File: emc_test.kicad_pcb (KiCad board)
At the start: 2 copper layers, 102 x 57 mm, 42 parts, among them X1 NEU, X2 LINE, X3 PE, X4 LINE, X5 PE, X6 NEU

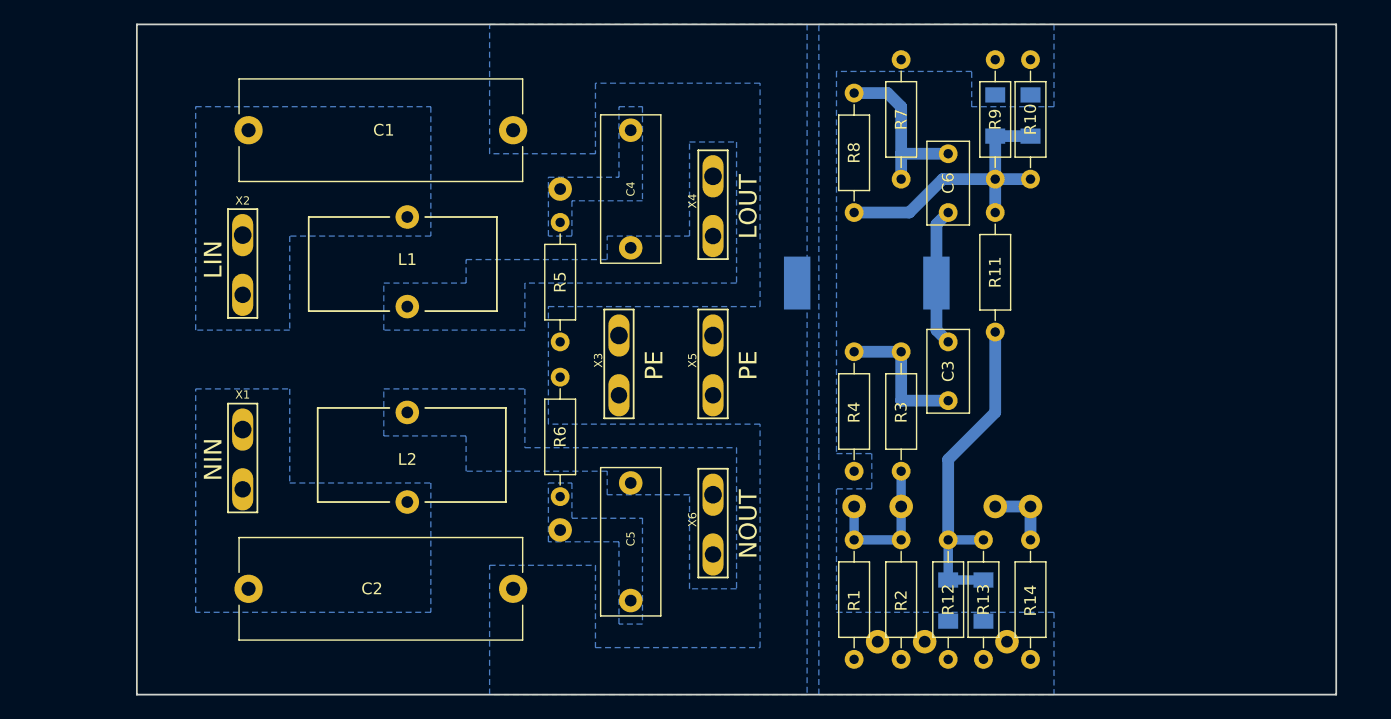
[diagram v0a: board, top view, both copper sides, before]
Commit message: plokstes paruosimas
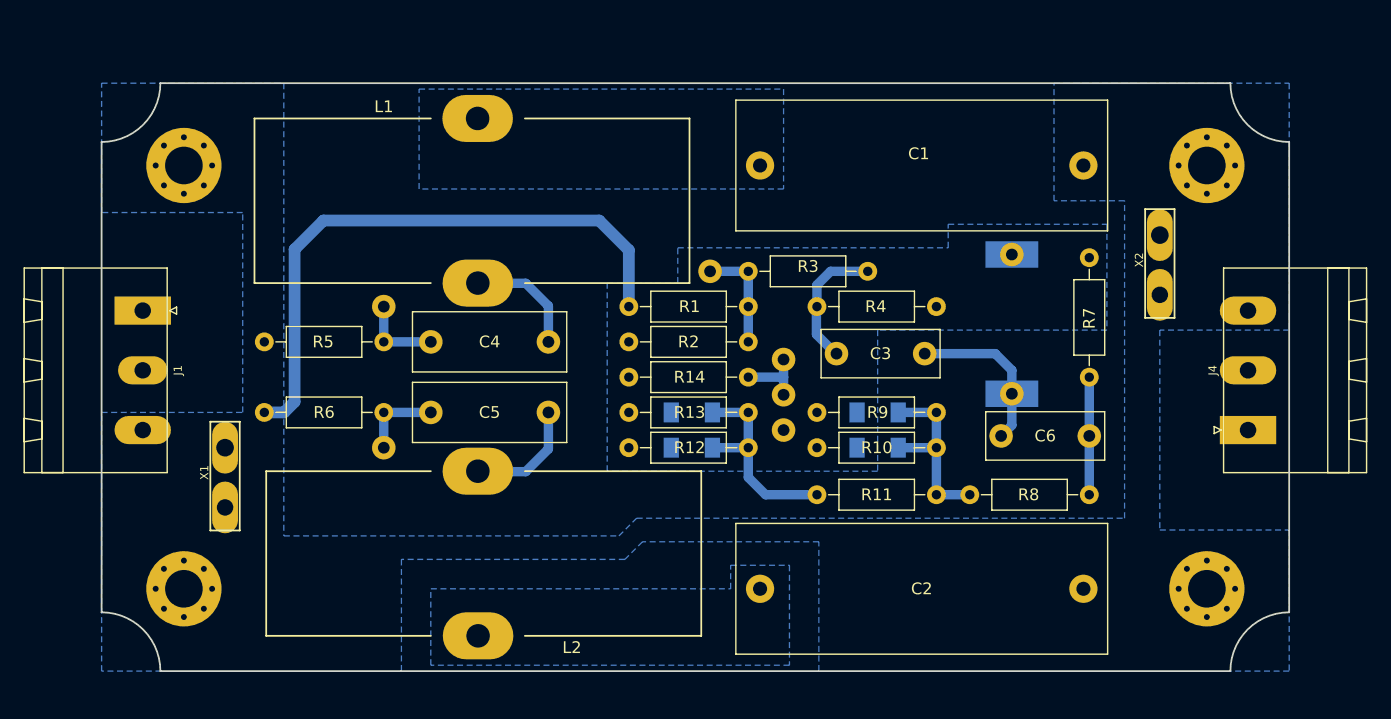
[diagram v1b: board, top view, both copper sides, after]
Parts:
- removed the REF** at (164.0, 121.5)
- removed the REF** at (168.0, 121.5)
- removed the REF** at (175.0, 121.5)
- removed the REF** at (177.0, 110.0)
- removed the REF** at (174.0, 110.0)
- removed the REF** at (162.0, 110.0)
- removed the REF** at (166.0, 110.0)
- removed the REF** at (137.0, 112.0)
- removed the REF** at (137.0, 83.0)
- removed X3, X5: PE, mech:Faston_6.3x0.8x14
- removed X4: LINE, mech:Faston_6.3x0.8x14
- removed X6: NEU, mech:Faston_6.3x0.8x14
- added J1: MSTBA_3C_5.08_Angled, mech:PhoenixContact_MSTBA-G_03x5.08mm_Angled, F.Cu at (101.5, 93.3)
- added J4: MSTBA_3C_5.08_Angled, mech:PhoenixContact_MSTBA-G_03x5.08mm_Angled, F.Cu at (195.5, 103.5)
- added REF**: SolderWirePad_single_1mmDrill, Wire_Pads:SolderWirePad_single_1mmDrill, F.Cu at (149.8, 90.0)
- added REF**: MountingHole_3.2mm_M3_Pad_Via, Mounting_Holes:MountingHole_3.2mm_M3_Pad_Via, F.Cu at (192.0, 81.0)
- added REF**: MountingHole_3.2mm_M3_Pad_Via, Mounting_Holes:MountingHole_3.2mm_M3_Pad_Via, F.Cu at (105.0, 117.0)
- added REF**: MountingHole_3.2mm_M3_Pad_Via, Mounting_Holes:MountingHole_3.2mm_M3_Pad_Via, F.Cu at (105.0, 81.0)
- added REF**: SolderWirePad_single_1mmDrill, Wire_Pads:SolderWirePad_single_1mmDrill, F.Cu at (156.0, 103.5)
- added REF**: SolderWirePad_single_1mmDrill, Wire_Pads:SolderWirePad_single_1mmDrill, F.Cu at (156.0, 100.5)
- added REF**: SolderWirePad_single_1mmDrill, Wire_Pads:SolderWirePad_single_1mmDrill, F.Cu at (156.0, 97.5)
- added REF**: SolderWirePad_single_1mmDrill, Wire_Pads:SolderWirePad_single_1mmDrill, F.Cu at (122.0, 105.0)
- added REF**: SolderWirePad_single_1mmDrill, Wire_Pads:SolderWirePad_single_1mmDrill, F.Cu at (122.0, 93.0)
- added REF**: SolderWirePad_single_1mmDrill, Wire_Pads:SolderWirePad_single_1mmDrill, F.Cu at (175.4, 100.4)
- added REF**: SolderWirePad_single_1mmDrill, Wire_Pads:SolderWirePad_single_1mmDrill, F.Cu at (175.4, 88.6)
- added REF**: MountingHole_3.2mm_M3_Pad_Via, Mounting_Holes:MountingHole_3.2mm_M3_Pad_Via, F.Cu at (192.0, 117.0)
- C1, C2: footprint Capacitors_THT:C_Rect_L24.0mm_W8.6mm_P22.50mm_MKT -> Capacitors_THT:C_Rect_L31.5mm_W11.0mm_P27.50mm_MKS4
- C3, C6: footprint Capacitors_THT:C_Rect_L7.0mm_W3.5mm_P5.00mm -> Capacitors_THT:C_Rect_L10.0mm_W4.0mm_P7.50mm_MKS4
- C4, C5: footprint capacitors:C_Disc_D12.5mm_W5.0mm_P10.00mm -> Capacitors_THT:C_Rect_L13.0mm_W5.0mm_P10.00mm_FKS3_FKP3_MKS4
- L1, L2: footprint Choke_Toroid_ThroughHole:Choke_Toroid_8x16mm_Vertical -> disc:Choke_Toroid_12x38mm_Vertical
- R1, R10, R11, R12, R13, R14, R2, R3, R4, R7, R8, R9: footprint resistors:R_Axial_DIN0207_L6.3mm_D2.5mm_P10.16mm_Horizontal -> Resistors_THT:R_Axial_DIN0207_L6.3mm_D2.5mm_P10.16mm_Horizontal
- X1: value NEU -> PE
- X2: value LINE -> PE
- moved X2 78.0 mm to (188.0, 89.5)
- moved C2 48.5 mm to (181.5, 117.0)
- moved C1 43.6 mm to (154.0, 81.0)
- moved R14 41.7 mm to (142.8, 99.0), turned to 0 degrees
- moved R8 39.6 mm to (182.0, 109.0), turned to 180 degrees
- moved R10 37.7 mm to (158.8, 105.0), turned to 0 degrees
- moved R13 36.8 mm to (142.8, 102.0), turned to 0 degrees
- moved R1 35.6 mm to (142.8, 93.0), turned to 0 degrees
- moved R2 35.6 mm to (142.8, 96.0), turned to 0 degrees
- moved R9 33.6 mm to (158.8, 102.0), turned to 0 degrees
- moved R12 32.6 mm to (142.8, 105.0), turned to 0 degrees
- moved D1 31.1 mm to (164.0, 105.0), turned to 180 degrees
- moved D4 28.0 mm to (148.2, 105.0), turned to 0 degrees
- moved D2 27.2 mm to (164.0, 102.0), turned to 0 degrees
- moved D3 27.0 mm to (148.2, 102.0), turned to 180 degrees
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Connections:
- X1 pad 1: /NEU -> Earth
- X2 pad 1: /LINE -> Earth
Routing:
- net Earth: track 0.00 -> 51.2 mm
- net Net-(D3-Pad1): track 28.7 -> 18.1 mm
- net Net-(C5-Pad2): track 0.00 -> 9.91 mm
- net Net-(C4-Pad1): track 0.00 -> 9.89 mm
- net Net-(D1-Pad1): track 25.7 -> 16.3 mm
- net Net-(C5-Pad1): track 0.00 -> 7.00 mm
- net Net-(C4-Pad2): track 0.00 -> 7.00 mm
- net Net-(C6-Pad2): track 14.7 -> 10.0 mm
- net Net-(R1-Pad2): track 12.7 -> 9.25 mm
- net Net-(C3-Pad2): track 11.8 -> 14.0 mm
- net Net-(C3-Pad1): track 12.2 -> 11.3 mm
- removed copper zone on B.Cu, net Net-(C4-Pad1)
- removed copper zone on B.Cu, net Net-(C4-Pad2)
- removed copper zone on B.Cu, net Net-(C5-Pad1)
- removed copper zone on B.Cu, net Net-(C5-Pad2)
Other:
- board size 102 x 57 mm -> 101 x 50 mm
- board text removed: "LIN"
- board text removed: "LOUT"
- board text removed: "NIN"
- board text removed: "NOUT"
- board text removed: "PE"
